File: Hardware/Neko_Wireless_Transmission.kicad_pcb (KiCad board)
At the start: 4 copper layers, 27.1 x 27 mm, 48 parts, among them IC1 W25Q32JVSSIQ, IC2 ESP32-D0WD, IC3 IPS6404L-SQ-SPN, J1 OV2640, Q1 AO3401A, U1 XC6206P282MR, U2 XC6206P122MR, Y1 YSX321SL_40Mhz

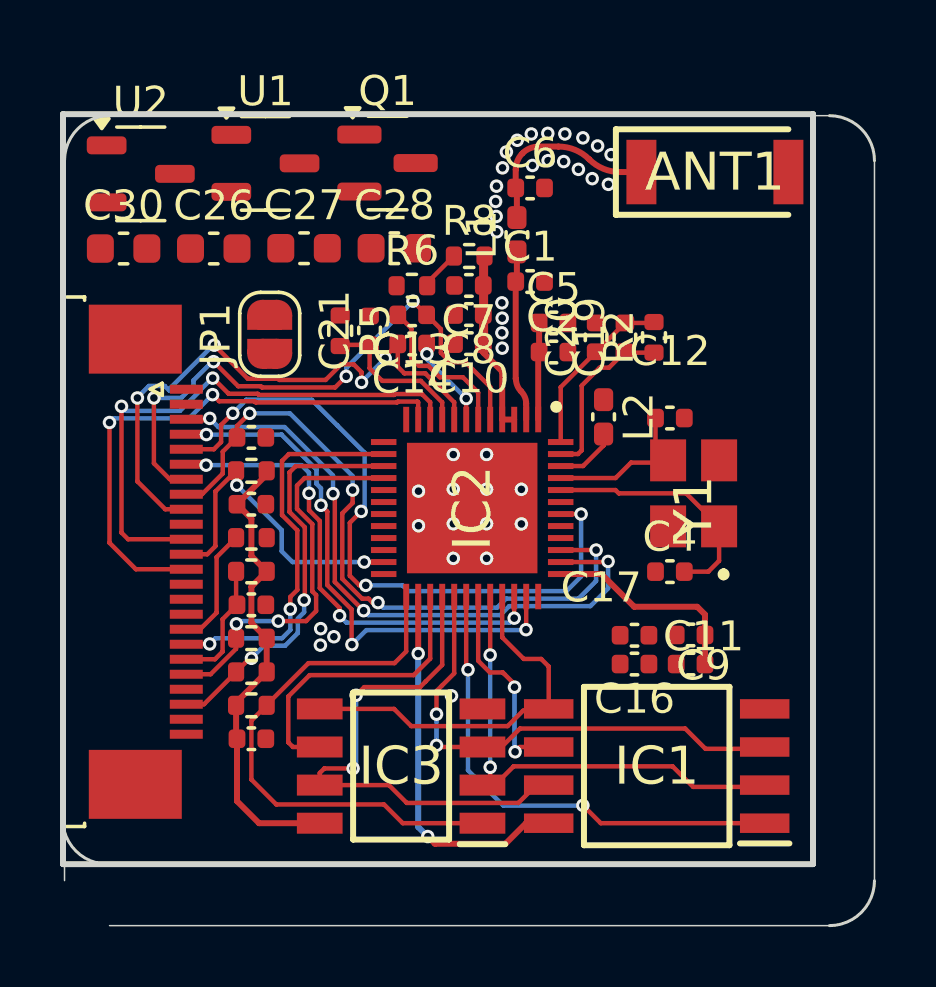
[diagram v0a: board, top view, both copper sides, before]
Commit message: Update New PCB Layput
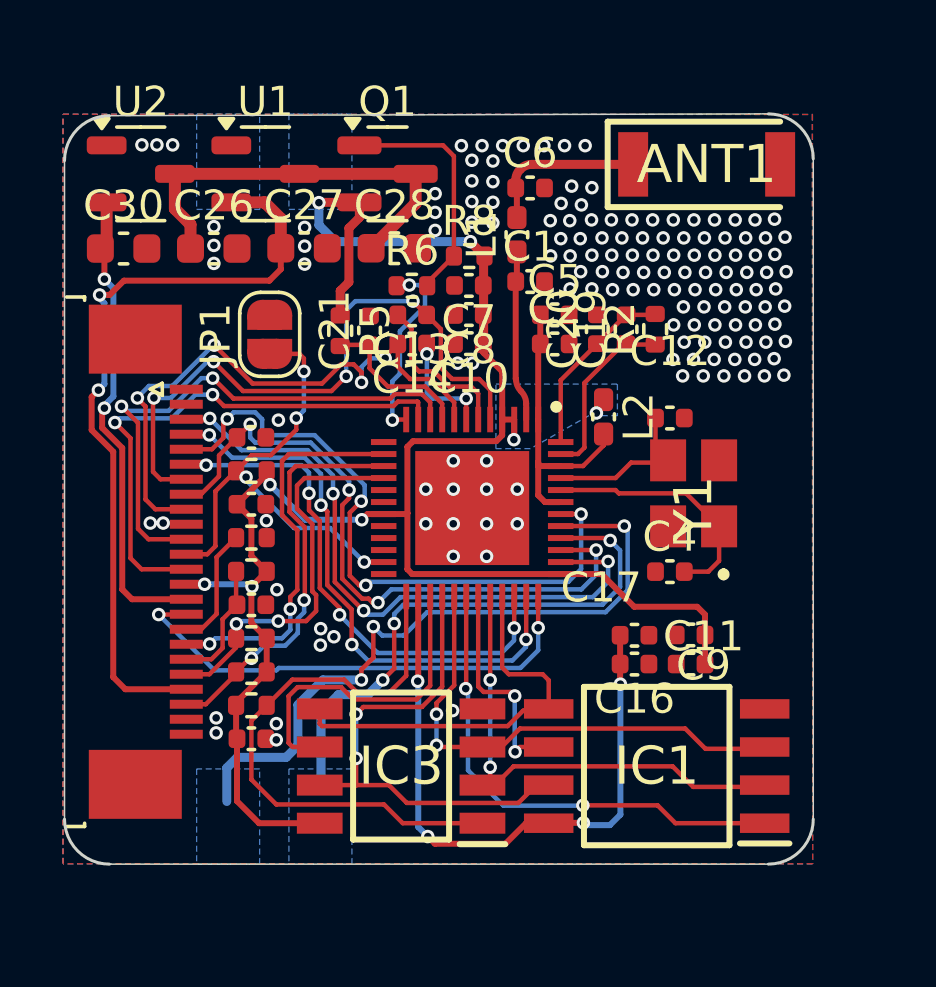
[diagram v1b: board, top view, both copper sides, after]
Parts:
- moved ANT1 0.38 mm to (45.2, 64.5)
- moved Q1 0.36 mm to (34.5, 64.8)
- moved U1 0.35 mm to (30.5, 64.8)
- moved C2 0.27 mm to (40.1, 70.5)
- moved C5 0.27 mm to (40.1, 69.5)
- moved C19 0.27 mm to (42.5, 70.0)
- moved C20 0.27 mm to (41.5, 70.0)
- moved R2 0.27 mm to (43.5, 70.0)
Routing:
- net +3.3V: track 28.9 -> 63.2 mm, vias 0 -> 8
- net CSI_2.8V: track 0.00 -> 25.8 mm, vias 0 -> 2
- net /U0TXD: track 0.00 -> 23.1 mm, vias 0 -> 3
- net /U0RXD: track 0.00 -> 18.6 mm, vias 0 -> 3
- net /CSI_HSYNC: track 0.00 -> 16.4 mm, vias 0 -> 2
- net CSI_1.8V: track 0.00 -> 15.9 mm, vias 0 -> 2
- net CAM_3.3V: track 0.00 -> 13.8 mm
- net VDD_SDIO: track 12.5 -> 21.1 mm, vias 2 -> 4
- net Net-(Q1-G): track 1.36 -> 7.99 mm
- net /CAM_PWR: track 0.00 -> 6.27 mm, vias 0 -> 2
- net /CSI_MCLK: track 10.7 -> 16.4 mm, vias 2 -> 4
- net +3.3VADC: track 5.33 -> 9.86 mm
- net /CSI_D4: track 19.7 -> 21.3 mm
- net /CSI_D0: track 16.1 -> 17.3 mm
- net /CSI_D3: track 22.9 -> 21.8 mm
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- added copper zone on B.Cu, net +3.3V
- added copper zone on B.Cu, net /U0RXD
- added copper zone on B.Cu, net /U0TXD
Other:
- board size 27.1 x 27 mm -> 25 x 25 mm
- copper layers 4 -> 2
